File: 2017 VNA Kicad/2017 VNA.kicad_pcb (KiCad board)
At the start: 2 copper layers, 50 x 30 mm, 49 parts, among them P1 Output, P2 Input, U1 SI5351A, U2 NL7WB66, U3 NL7WB66, Y1 CX3225

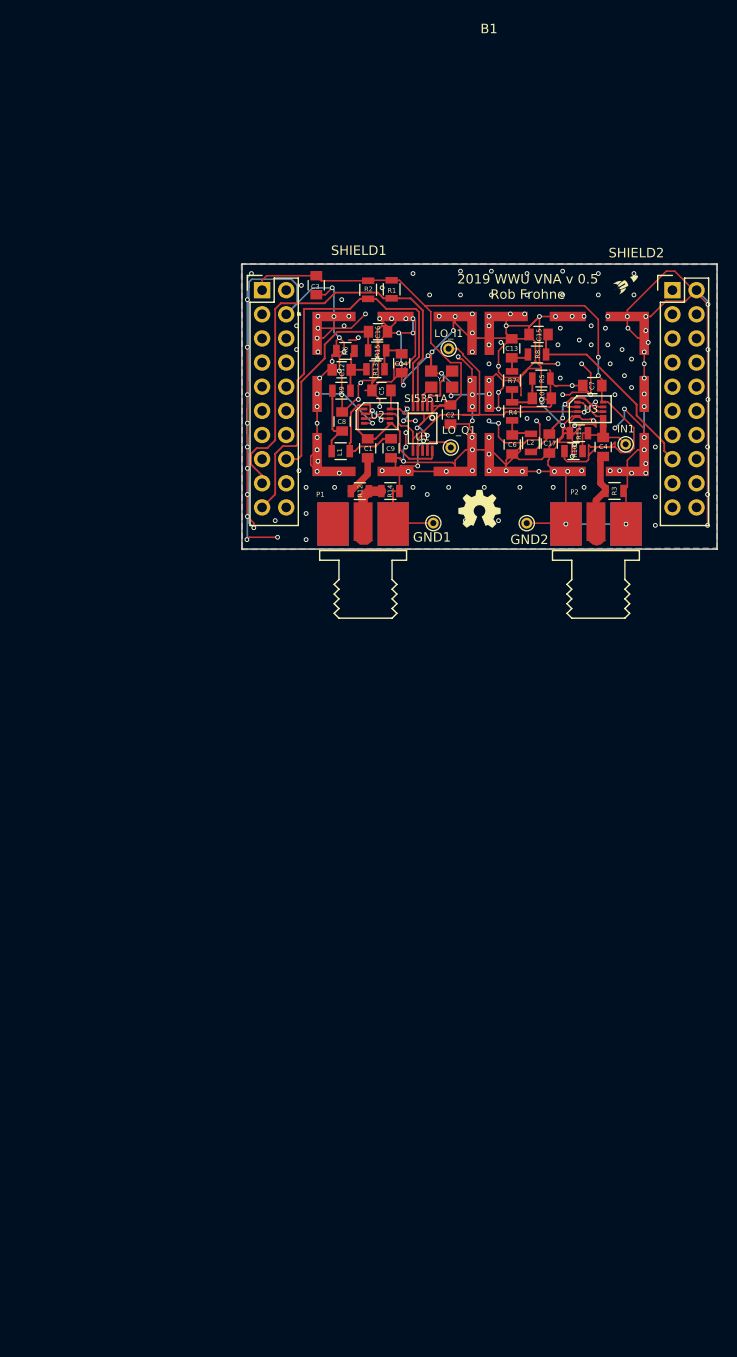
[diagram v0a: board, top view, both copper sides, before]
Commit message: New PCB spin.
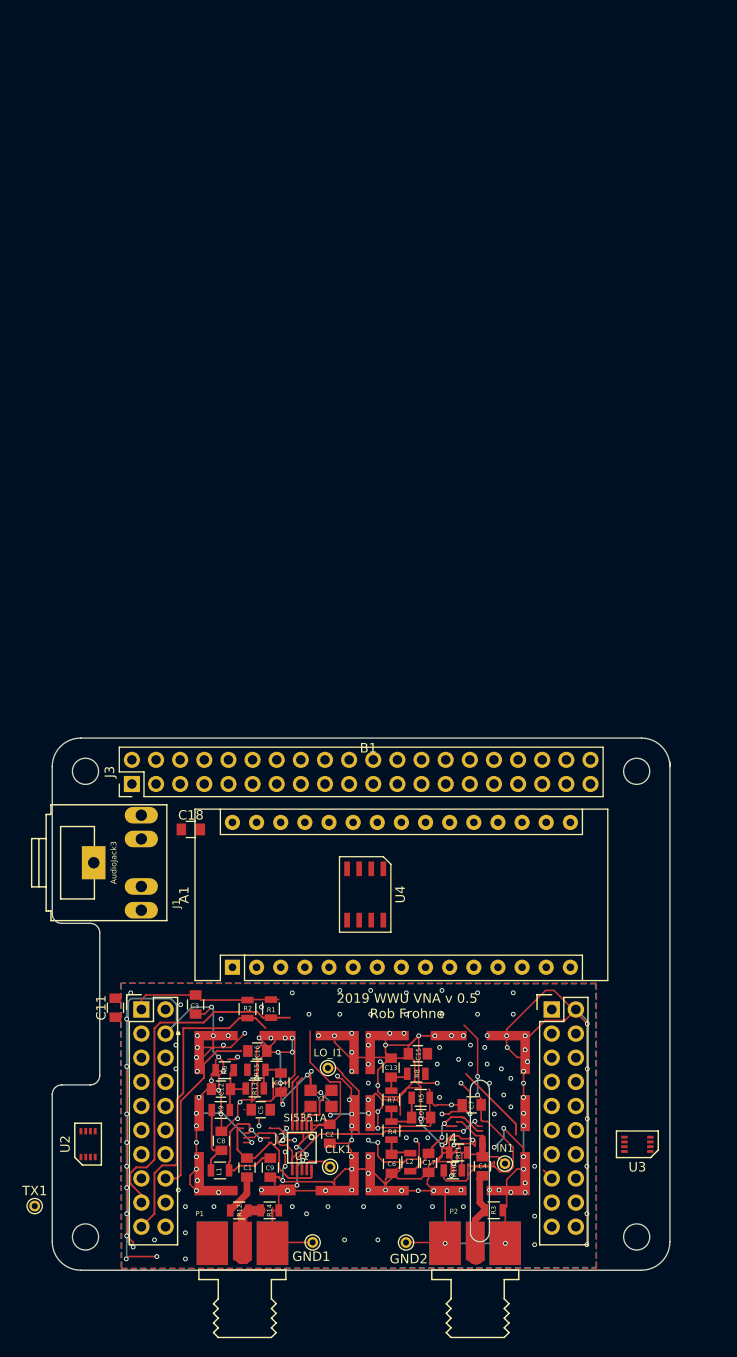
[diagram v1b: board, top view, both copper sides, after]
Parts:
- removed G***: Launchpad_LOGO_small, kilibs:Launchpad_LOGO_small
- removed G***: LOGO, EtherkitKicadLibrary:OSHWLogo4mm
- removed SHIELD1, SHIELD2: BMI-S-202-F, kilibs:LAIRD-BMI-S-202
- added ?: , RPi_Hat:RPi_Hat_Mounting_Hole, F.Cu at (111.5, 172.4)
- added ?: , RPi_Hat:RPi_Hat_Mounting_Hole, F.Cu at (111.5, 123.4)
- added ?: , RPi_Hat:RPi_Hat_Mounting_Hole, F.Cu at (53.5, 123.4)
- added ?: , RPi_Hat:RPi_Hat_Mounting_Hole, F.Cu at (53.5, 172.4)
- added A1: Arduino_Nano_v3.x, Modules:Arduino_Nano, F.Cu at (69.0, 144.0)
- added C11: 0.1uF, Capacitors_SMD:C_0805, F.Cu at (56.7, 148.3)
- added C18: 0.1uF, Capacitors_SMD:C_0805, F.Cu at (64.6, 129.5)
- added J1: AudioJack3, 2017 VNA Kicad:Tayda_3.5mm_stereo_TRS_jack_A-853, F.Cu at (56.0, 133.0)
- added J2: RF_Shield_Two_Pieces, kilibs:LAIRD-BMI-S-202, F.Cu at (65.0, 168.0)
- added J3: Raspberry_Pi_2_3, Pin_Headers:Pin_Header_Straight_2x20_Pitch2.54mm, F.Cu at (58.4, 124.7)
- added J4: RF_Shield_Two_Pieces, kilibs:LAIRD-BMI-S-202, F.Cu at (83.0, 168.0)
- added TX1: LO_Q, Connectors:PINTST, F.Cu at (48.2, 169.1)
- added U4: LM2904, 2017 VNA Kicad:SOIC-8, F.Cu at (83.0, 136.3)
- R3: value 56 -> 47
- moved U2 82.4 mm to (53.8, 162.6), turned to 0 degrees
- moved U3 77.5 mm to (111.6, 162.6), turned to 90 degrees
- moved B1 76.8 mm to (83.5, 148.4)
- moved C10 76.8 mm to (88.9, 159.8)
- moved C12 76.8 mm to (67.8, 156.8)
- moved C13 76.8 mm to (85.7, 154.6)
- moved C14 76.8 mm to (74.1, 156.1)
- moved C15 76.8 mm to (88.5, 153.1)
- moved C16 76.8 mm to (71.6, 152.8)
- moved C4 76.8 mm to (95.3, 164.9)
- moved C8 76.8 mm to (67.8, 162.3)
- moved CLK1 76.8 mm to (79.3, 165.0)
- moved IN1 76.8 mm to (97.7, 164.7)
- moved L1 76.8 mm to (67.7, 165.4)
- moved L2 76.8 mm to (87.7, 164.5)
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- renumbered LO_Q1 to CLK1
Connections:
- B1 pad 5V: (no net) -> +5V
- C1 pad 2: /Ref_In -> /TX
- C15 pad 1: Net-(B1-PadP5.1) -> Net-(C15-Pad1)
- C16 pad 1: Net-(B1-PadP4.7) -> Net-(C16-Pad1)
- C5 pad 1: +3V3 -> GND
- C5 pad 2: GND -> +3V3
- CLK1 pad 1: /LO_Q -> /Ref_In
- R15 pad 1: Net-(B1-PadP4.7) -> Net-(C16-Pad1)
- R8 pad 1: Net-(B1-PadP5.1) -> Net-(C15-Pad1)
- U1 pad 10: /Ref_In -> /TX
- U1 pad 9: /LO_Q -> /Ref_In
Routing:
- net +3V3: track 102.8 -> 79.4 mm
- net /TX: track 0.00 -> 15.1 mm
- net /Ref_In: track 15.1 -> 3.46 mm
- net Net-(B1-PadP5.1): track 21.2 -> 9.81 mm
- net GND: track 544.7 -> 535.0 mm, vias 196 -> 192
- net /SDA: track 46.8 -> 38.5 mm
- net /SCL: track 47.8 -> 40.9 mm
- net /LO_Q: track 3.46 -> 0.00 mm
- net Net-(B1-PadP4.7): track 21.6 -> 18.9 mm
- net /LO_I: vias 2 -> 3
- net Net-(C9-Pad1): vias 2 -> 3
- net (no net): vias 4 -> 5
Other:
- board size 50 x 30 mm -> 65 x 56 mm
- board text added: "Camera Flex Slot (Optional)"
- board text added: "Dimensions taken from https://github.com/raspberrypi/hats/blob/master/hat-board-mechanical.pdf"
